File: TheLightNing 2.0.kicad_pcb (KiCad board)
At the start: 2 copper layers, 75 x 60 mm, 27 parts, among them J1 motores izq, J2 motores der, J3 batt, J4 LED_izq, J5 salida a modulo, SW1 SW_SPDT, U1 L298(H)N, U2 ESP32_DEVKITC, U3 L7805

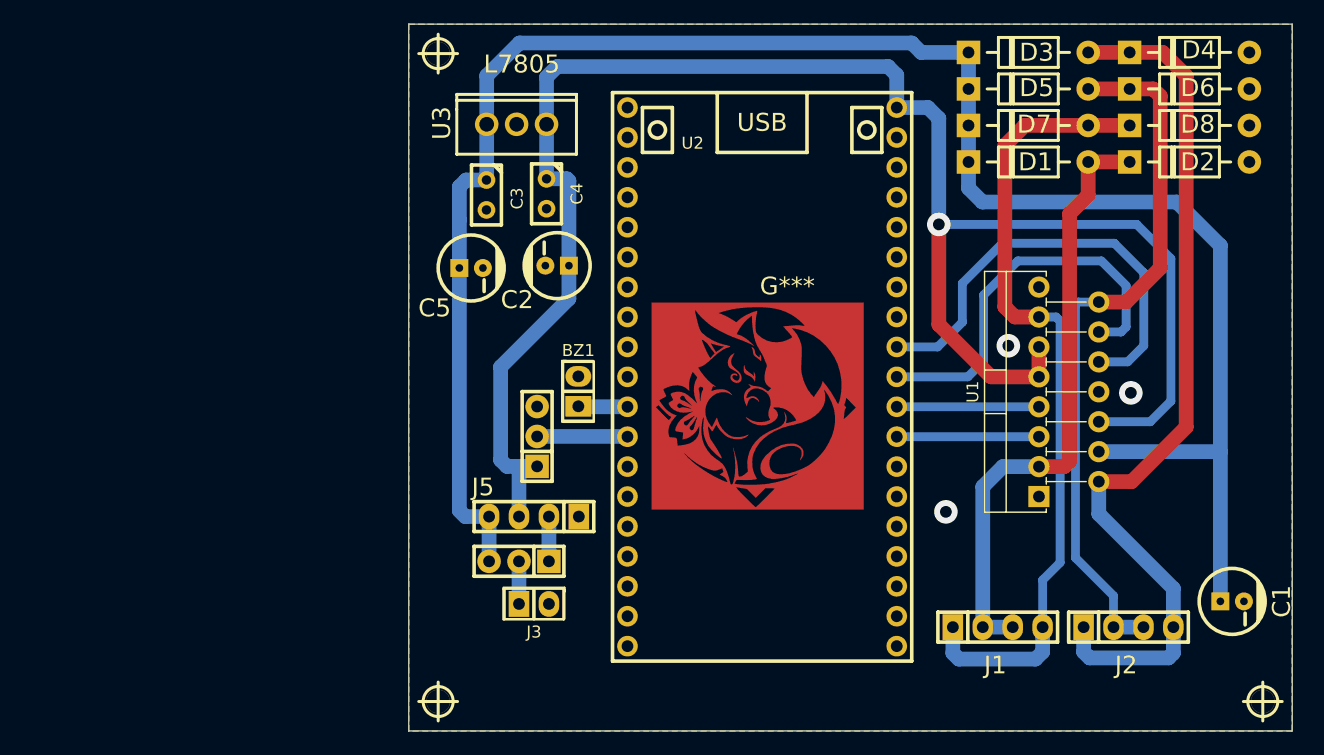
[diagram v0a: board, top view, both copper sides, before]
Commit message: rework
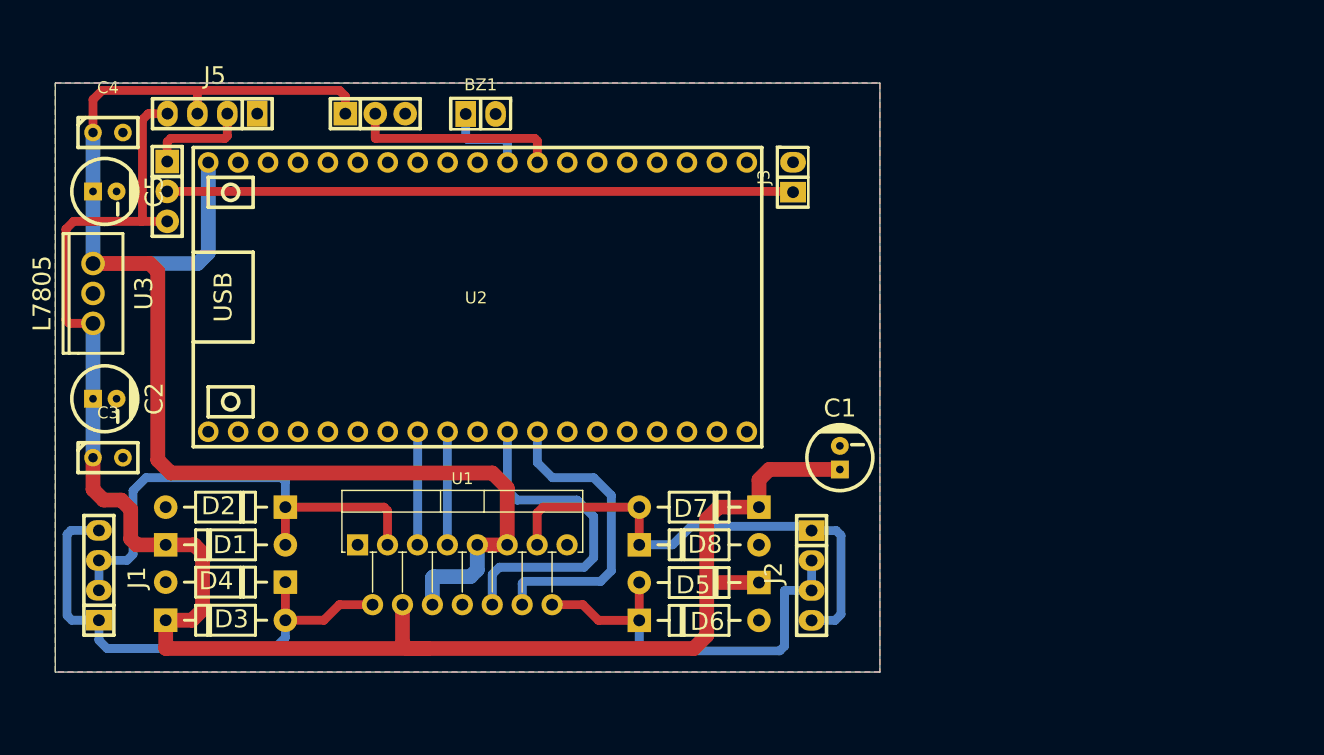
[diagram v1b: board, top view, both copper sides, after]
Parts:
- removed G***: LOGO, logo:yae
- removed hole_2mm (x3): VAL**, EESTN5:hole_2mm
- moved D4 93.4 mm to (99.5, 87.4), turned to 0 degrees
- moved D2 86.9 mm to (99.5, 81.0), turned to 0 degrees
- moved D3 83.5 mm to (99.5, 90.6)
- moved J1 76.4 mm to (88.7, 86.8), turned to 90 degrees
- moved D1 75.5 mm to (99.5, 84.2)
- moved D6 61.4 mm to (139.7, 90.6)
- moved U1 58.0 mm to (110.7, 84.2), turned to 0 degrees
- moved D8 54.8 mm to (139.7, 84.2)
- moved D5 50.4 mm to (139.7, 87.4), turned to 0 degrees
- moved J5 43.8 mm to (98.3, 47.6)
- moved SW1 43.3 mm to (94.5, 54.2), turned to -90 degrees
- moved D7 42.8 mm to (139.7, 81.0), turned to 0 degrees
- moved J3 41.9 mm to (147.3, 53.0), turned to 90 degrees
- moved C3 39.1 mm to (89.5, 76.8), turned to 0 degrees
- moved C5 38.9 mm to (89.2, 54.2), turned to -90 degrees
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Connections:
- J1 pad 1: Net-(D7-A) -> Net-(D3-A)
- J1 pad 4: Net-(D7-A) -> Net-(D3-A)
- J2 pad 1: Net-(D3-A) -> Net-(D7-A)
- J2 pad 4: Net-(D3-A) -> Net-(D7-A)
- U2 pad 10: /IN4 -> unconnected-(U2-IO26-Pad10)
- U2 pad 11: /IN3 -> unconnected-(U2-IO27-Pad11)
- U2 pad 27: unconnected-(U2-IO16-Pad27) -> /IN1
- U2 pad 28: unconnected-(U2-IO17-Pad28) -> /IN2
- U2 pad 30: /buzz -> /IN3
- U2 pad 31: /led -> /IN4
- U2 pad 8: /IN1 -> /led
- U2 pad 9: /IN2 -> /buzz
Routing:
- net Net-(SW1-B): track 3.62 -> 53.2 mm
- net Net-(D3-A): track 75.6 -> 43.5 mm
- net Net-(D7-A): track 69.2 -> 42.3 mm
- net +5V: track 151.8 -> 125.5 mm, vias 1 -> 0
- net Net-(D5-A): track 60.7 -> 35.5 mm
- net VCC: track 163.3 -> 149.7 mm
- net Net-(D1-A): track 52.3 -> 41.6 mm
- net /led: track 7.68 -> 17.7 mm
- net /IN3: track 38.2 -> 28.5 mm
- net /IN4: track 33.7 -> 26.3 mm
- net /Cargador: track 3.80 -> 8.87 mm
- net /buzz: track 4.19 -> 7.40 mm
- net /IN2: track 12.1 -> 9.61 mm
- net /IN1: track 12.1 -> 9.64 mm
- net GND: vias 3 -> 0
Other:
- board size 75 x 60 mm -> 70 x 50 mm
